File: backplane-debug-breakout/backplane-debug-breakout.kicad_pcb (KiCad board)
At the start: 2 copper layers, 65 x 51.9 mm, 15 parts, among them J1 Conn_02x08_Odd_Even, J2 Conn_01x04, J3 Conn_01x01_Socket, J4 Conn_01x01_Socket, J5 Conn_01x04, J6 629105150521, SW1 SW_Push_DPDT, SW2 SW_Omron_B3FS, SW3 EG1218, U1 UMFT234XF

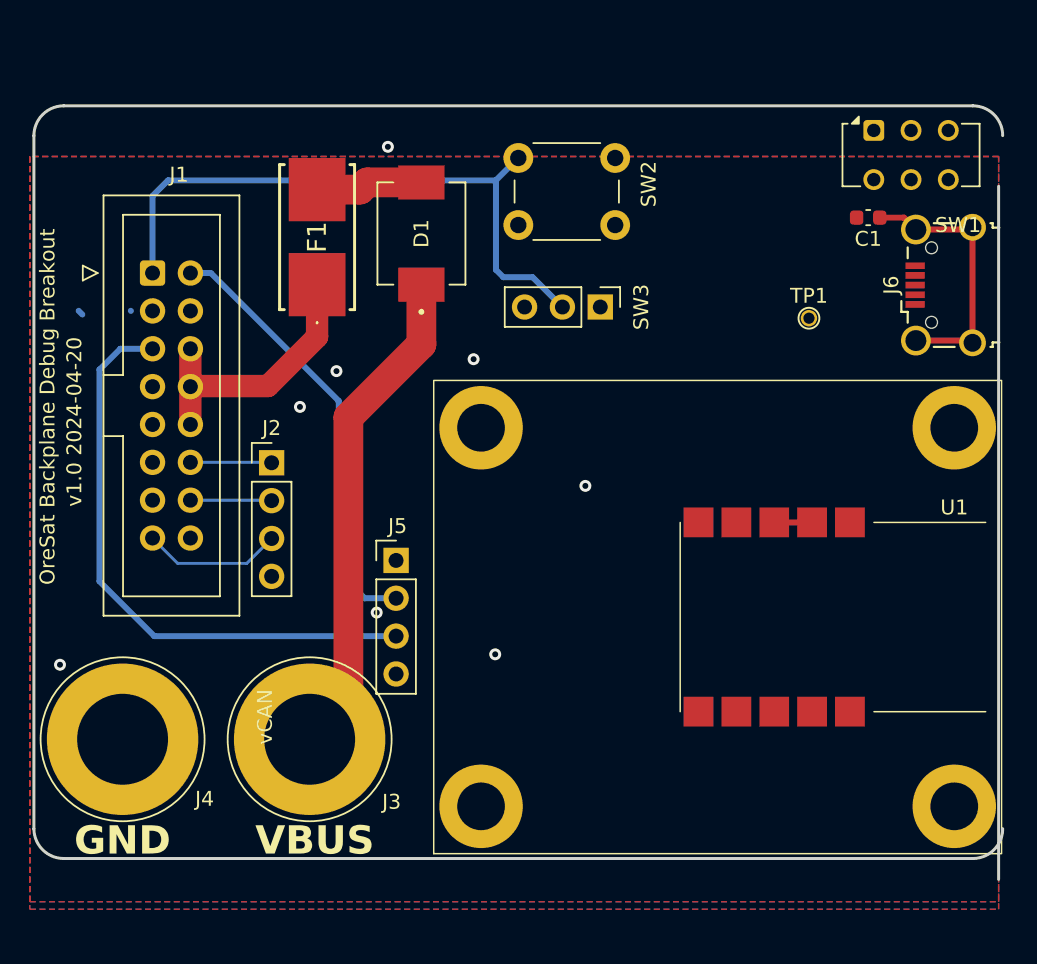
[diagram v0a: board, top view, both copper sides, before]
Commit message: made changes to layout of pcb
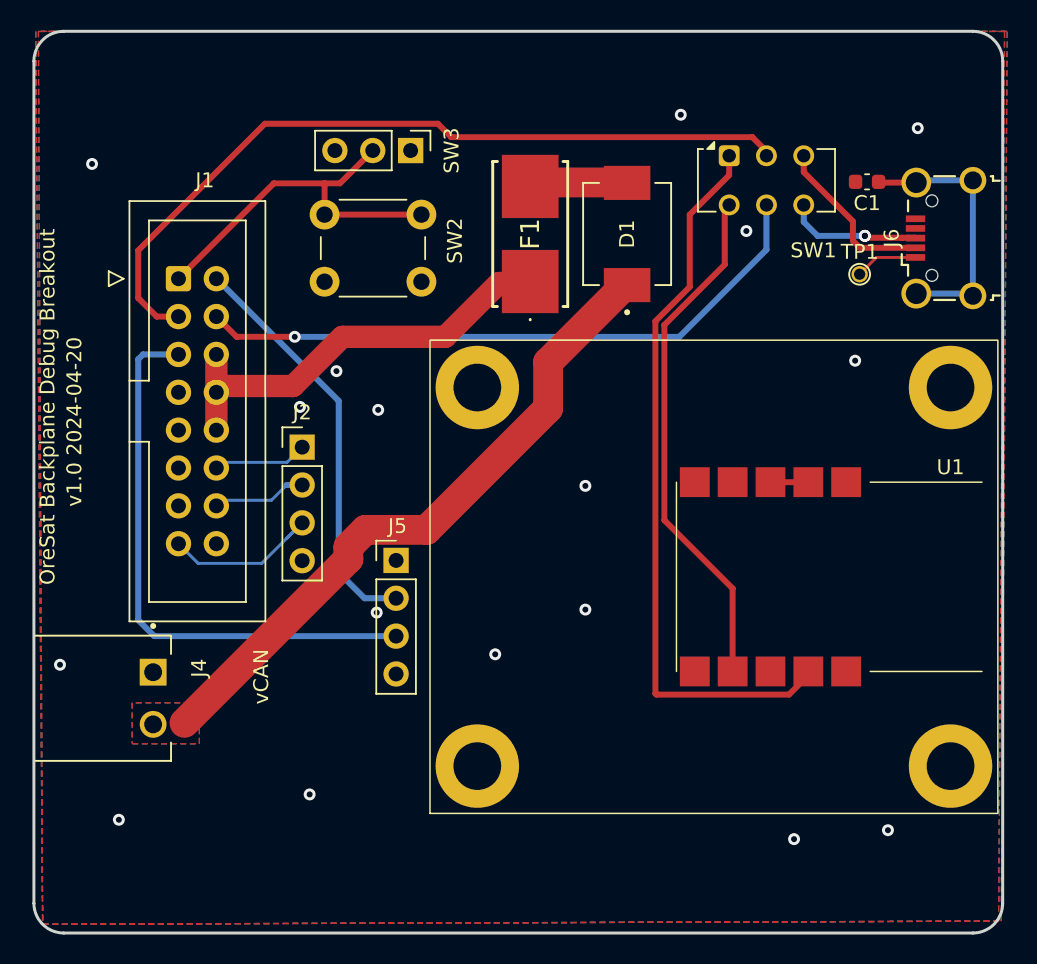
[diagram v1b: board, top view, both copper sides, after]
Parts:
- removed J3: Conn_01x01_Socket, Connector:Banana_Jack_1Pin
- J4: value Conn_01x01_Socket -> Conn_01x02_Socket; footprint Connector:Banana_Jack_1Pin -> oresat-connectors:PHOENIX_1995499
- moved SW3 16.5 mm to (122.3, 62.0)
- moved F1 14.3 mm to (130.3, 67.6)
- moved D1 13.8 mm to (136.8, 67.6)
- moved SW2 13.5 mm to (123.0, 70.8)
- moved SW1 9.85 mm to (149.3, 69.2)
- moved J4 9.15 mm to (97.0, 94.5)
- moved TP1 4.50 mm to (152.4, 70.3)
- moved J6 3.15 mm to (158.1, 67.9)
- moved U1 2.71 mm to (161.1, 84.2)
- moved vCAN 2.71 mm to (126.8, 103.3)
- moved C1 2.40 mm to (152.9, 64.1)
- moved J2 2.30 mm to (115.0, 81.9)
- moved J1 1.78 mm to (106.7, 70.6)
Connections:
- J4 pad 1: GND -> Net-(D1-A)
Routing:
- net /C3-UART-TX: track 0.37 -> 53.2 mm
- net Net-(U1-RXD): track 0.26 -> 49.2 mm
- net /C3-UART-RX: track 0.00 -> 42.9 mm, vias 0 -> 1
- net Net-(U1-TXD): track 0.00 -> 35.0 mm
- net /SD: track 42.3 -> 25.2 mm
- net Net-(J6-D-): track 0.00 -> 11.5 mm
- net /VBUS: track 18.5 -> 29.2 mm
- net Net-(D1-A): track 34.3 -> 44.2 mm
- net Net-(J6-D+): track 0.00 -> 9.10 mm, vias 0 -> 2
- net Net-(J6-VBUS): track 0.00 -> 4.22 mm
- net /CAN_L: track 29.6 -> 27.7 mm
- net /CAN_H: track 39.8 -> 38.1 mm
- net /OPD_SCL: track 9.87 -> 11.5 mm
- net /OPD_PWR: track 5.46 -> 6.35 mm
- net /OPD_SDA: track 5.46 -> 6.34 mm
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- added copper zone on B.Cu, net Net-(D1-A)
- added copper zone on F.Cu, net Net-(D1-A)
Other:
- board size 65 x 51.9 mm -> 65 x 60.5 mm
- board text removed: "GND"
- board text removed: "VBUS"
